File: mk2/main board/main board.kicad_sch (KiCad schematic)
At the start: 6 parts, among them J1 Conn_01x02_Male, Q1 IRLZ44N

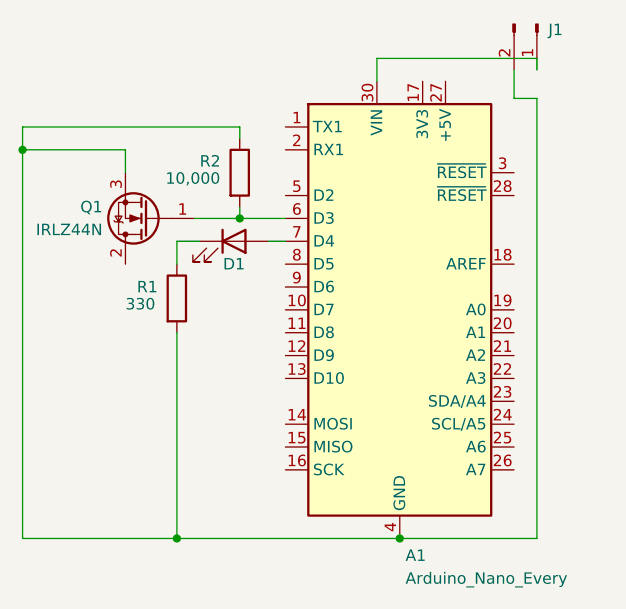
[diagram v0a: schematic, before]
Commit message: PCB Updates
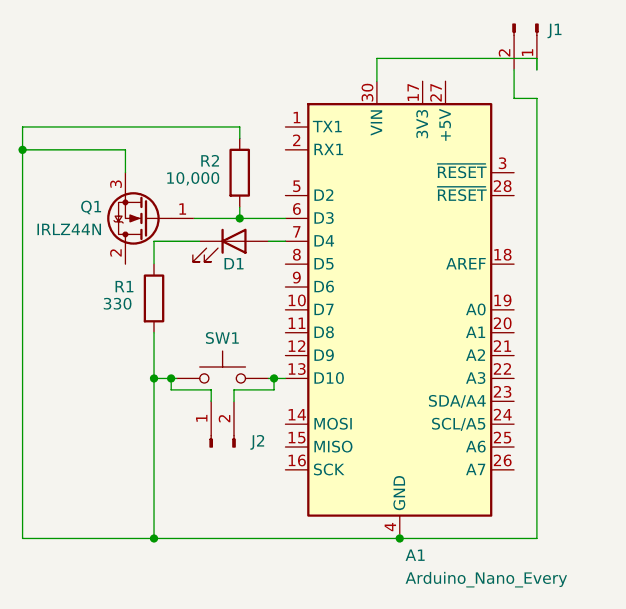
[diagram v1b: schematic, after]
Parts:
- added J2: Conn_01x02_Male, Connector_PinHeader_2.54mm:PinHeader_1x02_P2.54mm_Horizontal, symbol Connector:Conn_01x02_Male
- added SW1: SW_Push, Button_Switch_THT:SW_PUSH-12mm, symbol Switch:SW_Push
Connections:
- net at A1.13 (D10): now also J2.2 (Pin_2), SW1.2
- net at A1.29 (GND), A1.4 (GND), J1.2 (Pin_2)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: now also J2.1 (Pin_1), SW1.1
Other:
- moved on the sheet: R1
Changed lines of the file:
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@@
   (junction (at 116.84 89.535) (diameter 0) (color 0 0 0 0)
   )
-  (junction (at 133.985 132.715) (diameter 0) (color 0 0 0 0)
+  (junction (at 144.78 114.935) (diameter 0) (color 0 0 0 0)
+  )
+  (junction (at 131.445 132.715) (diameter 0) (color 0 0 0 0)
   )
   (junction (at 158.75 132.715) (diameter 0) (color 0 0 0 0)
   )
+  (junction (at 133.35 114.935) (diameter 0) (color 0 0 0 0)
+  )
+  (junction (at 131.445 114.935) (diameter 0) (color 0 0 0 0)
+  )
   (junction (at 140.97 97.155) (diameter 0) (color 0 0 0 0)
   )
-  (wire (pts (xy 133.985 99.695) (xy 133.985 102.235))
+  (wire (pts (xy 131.445 99.695) (xy 131.445 102.235))
     (stroke (width 0) (type default) (color 0 0 0 0))
   )
@@
     (stroke (width 0) (type default) (color 0 0 0 0))
   )
+  (wire (pts (xy 131.445 114.935) (xy 133.35 114.935))
+    (stroke (width 0) (type default) (color 0 0 0 0))
+  )
   (wire (pts (xy 135.89 97.155) (xy 140.97 97.155))
     (stroke (width 0) (type default) (color 0 0 0 0))
@@
     (stroke (width 0) (type default) (color 0 0 0 0))
   )
-  (wire (pts (xy 133.985 109.855) (xy 133.985 132.715))
+  (wire (pts (xy 131.445 109.855) (xy 131.445 114.935))
+    (stroke (width 0) (type default) (color 0 0 0 0))
+  )
+  (wire (pts (xy 140.335 117.475) (xy 140.335 116.205))
     (stroke (width 0) (type default) (color 0 0 0 0))
   )
@@
     (stroke (width 0) (type default) (color 0 0 0 0))
   )
-  (wire (pts (xy 116.84 132.715) (xy 133.985 132.715))
+  (wire (pts (xy 144.78 116.205) (xy 144.78 114.935))
+    (stroke (width 0) (type default) (color 0 0 0 0))
+  )
+  (wire (pts (xy 133.35 114.935) (xy 133.985 114.935))
+    (stroke (width 0) (type default) (color 0 0 0 0))
+  )
+  (wire (pts (xy 140.335 116.205) (xy 144.78 116.205))
+    (stroke (width 0) (type default) (color 0 0 0 0))
+  )
+  (wire (pts (xy 116.84 132.715) (xy 131.445 132.715))
     (stroke (width 0) (type default) (color 0 0 0 0))
   )
@@
     (stroke (width 0) (type default) (color 0 0 0 0))
   )
-  (wire (pts (xy 133.985 132.715) (xy 158.75 132.715))
+  (wire (pts (xy 144.78 114.935) (xy 146.05 114.935))
+    (stroke (width 0) (type default) (color 0 0 0 0))
+  )
+  (wire (pts (xy 133.35 116.205) (xy 133.35 114.935))
+    (stroke (width 0) (type default) (color 0 0 0 0))
+  )
+  (wire (pts (xy 144.145 114.935) (xy 144.78 114.935))
+    (stroke (width 0) (type default) (color 0 0 0 0))
+  )
+  (wire (pts (xy 131.445 132.715) (xy 158.75 132.715))
+    (stroke (width 0) (type default) (color 0 0 0 0))
+  )
+  (wire (pts (xy 131.445 114.935) (xy 131.445 132.715))
+    (stroke (width 0) (type default) (color 0 0 0 0))
+  )
+  (wire (pts (xy 137.795 116.205) (xy 133.35 116.205))
+    (stroke (width 0) (type default) (color 0 0 0 0))
+  )
+  (wire (pts (xy 137.795 117.475) (xy 137.795 116.205))
     (stroke (width 0) (type default) (color 0 0 0 0))
   )
@@
     (stroke (width 0) (type default) (color 0 0 0 0))
   )
-  (wire (pts (xy 136.525 99.695) (xy 133.985 99.695))
+  (wire (pts (xy 131.445 99.695) (xy 136.525 99.695))
     (stroke (width 0) (type default) (color 0 0 0 0))
   )
@@
     (pin "2")
   )
+  (symbol (lib_id "Connector:Conn_01x02_Male") (at 137.795 122.555 90) (unit 1)
+    (in_bom yes) (on_board yes) (fields_autoplaced)
+    (property "Reference" "J2" (id 0) (at 142.24 121.9199 90)
+      (effects (font (size 1.27 1.27)) (justify right))
+    )
+    (property "Value" "Conn_01x02_Male" (id 1) (at 134.62 121.92 0)
+      (effects (font (size 1.27 1.27)) hide)
+    )
+    (property "Footprint" "Connector_PinHeader_2.54mm:PinHeader_1x02_P2.54mm_Horizontal" (id 2) (at 137.795 122.555 0)
+      (effects (font (size 1.27 1.27)) hide)
+    )
+    (property "Datasheet" "~" (id 3) (at 137.795 122.555 0)
+      (effects (font (size 1.27 1.27)) hide)
+    )
+    (pin "1")
+    (pin "2")
+  )
   (symbol (lib_id "Device:R") (at 140.97 92.075 0) (unit 1)
     (in_bom yes) (on_board yes)
@@
     (pin "2")
   )
-  (symbol (lib_id "Device:R") (at 133.985 106.045 0) (unit 1)
-    (in_bom yes) (on_board yes)
-    (property "Reference" "R1" (id 0) (at 129.54 104.775 0)
-      (effects (font (size 1.27 1.27)) (justify left))
-    )
-    (property "Value" "330" (id 1) (at 128.27 106.68 0)
-      (effects (font (size 1.27 1.27)) (justify left))
-    )
-    (property "Footprint" "Resistor_THT:R_Axial_DIN0207_L6.3mm_D2.5mm_P7.62mm_Horizontal" (id 2) (at 132.207 106.045 90)
-      (effects (font (size 1.27 1.27)) hide)
-    )
-    (property "Datasheet" "~" (id 3) (at 133.985 106.045 0)
+  (symbol (lib_id "Device:R") (at 131.445 106.045 0) (unit 1)
+    (in_bom yes) (on_board yes)
+    (property "Reference" "R1" (id 0) (at 127 104.775 0)
+      (effects (font (size 1.27 1.27)) (justify left))
+    )
+    (property "Value" "330" (id 1) (at 125.73 106.68 0)
+      (effects (font (size 1.27 1.27)) (justify left))
+    )
+    (property "Footprint" "Resistor_THT:R_Axial_DIN0207_L6.3mm_D2.5mm_P7.62mm_Horizontal" (id 2) (at 129.667 106.045 90)
+      (effects (font (size 1.27 1.27)) hide)
+    )
+    (property "Datasheet" "~" (id 3) (at 131.445 106.045 0)
+      (effects (font (size 1.27 1.27)) hide)
+    )
+    (pin "1")
+    (pin "2")
+  )
+  (symbol (lib_id "Switch:SW_Push") (at 139.065 114.935 0) (unit 1)
+    (in_bom yes) (on_board yes)
+    (property "Reference" "SW1" (id 0) (at 139.065 110.49 0))
+    (property "Value" "SW_Push" (id 1) (at 139.065 109.22 0)
+      (effects (font (size 1.27 1.27)) hide)
+    )
+    (property "Footprint" "Button_Switch_THT:SW_PUSH-12mm" (id 2) (at 139.065 109.855 0)
+      (effects (font (size 1.27 1.27)) hide)
+    )
+    (property "Datasheet" "~" (id 3) (at 139.065 109.855 0)
       (effects (font (size 1.27 1.27)) hide)
     )
@@
       (reference "J1") (unit 1) (value "Conn_01x02_Male") (footprint "Connector_PinHeader_2.54mm:PinHeader_1x02_P2.54mm_Horizontal")
     )
+    (path "/70035f6c-c2c4-4801-ac68-1bcfc3cbad1a"
+      (reference "J2") (unit 1) (value "Conn_01x02_Male") (footprint "Connector_PinHeader_2.54mm:PinHeader_1x02_P2.54mm_Horizontal")
+    )
     (path "/46c6bf57-1f0a-4e92-aaa8-60259a633ef8"
       (reference "Q1") (unit 1) (value "IRLZ44N") (footprint "Package_TO_SOT_THT:TO-220-3_Vertical")
@@
       (reference "R2") (unit 1) (value "10,000") (footprint "Resistor_THT:R_Axial_DIN0207_L6.3mm_D2.5mm_P7.62mm_Horizontal")
     )
-  )
+    (path "/f6662114-e94f-4466-8b01-5f4d76363a86"
+      (reference "SW1") (unit 1) (value "SW_Push") (footprint "Button_Switch_THT:SW_PUSH-12mm")
+    )
+  )

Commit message: Board Updates (Simplification)
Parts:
- D1: footprint LED_THT:LED_D3.0mm -> fab:LED_1206
- R1: footprint Resistor_THT:R_Axial_DIN0207_L6.3mm_D2.5mm_P7.62mm_Horizontal -> fab:R_1206
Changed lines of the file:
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@@
 			)
 		)
-		(property "Footprint" "LED_THT:LED_D3.0mm"
+		(property "Footprint" "fab:LED_1206"
 			(at 140.335 99.695 0)
 			(effects
@@
 			)
 		)
-		(property "Footprint" "Resistor_THT:R_Axial_DIN0207_L6.3mm_D2.5mm_P7.62mm_Horizontal"
+		(property "Footprint" "fab:R_1206"
 			(at 129.667 106.045 90)
 			(effects
